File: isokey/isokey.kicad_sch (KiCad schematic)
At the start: 77 parts, among them Q1 BSS138, U1 BlackPill_STLINK, U3 TLV73318PDBV

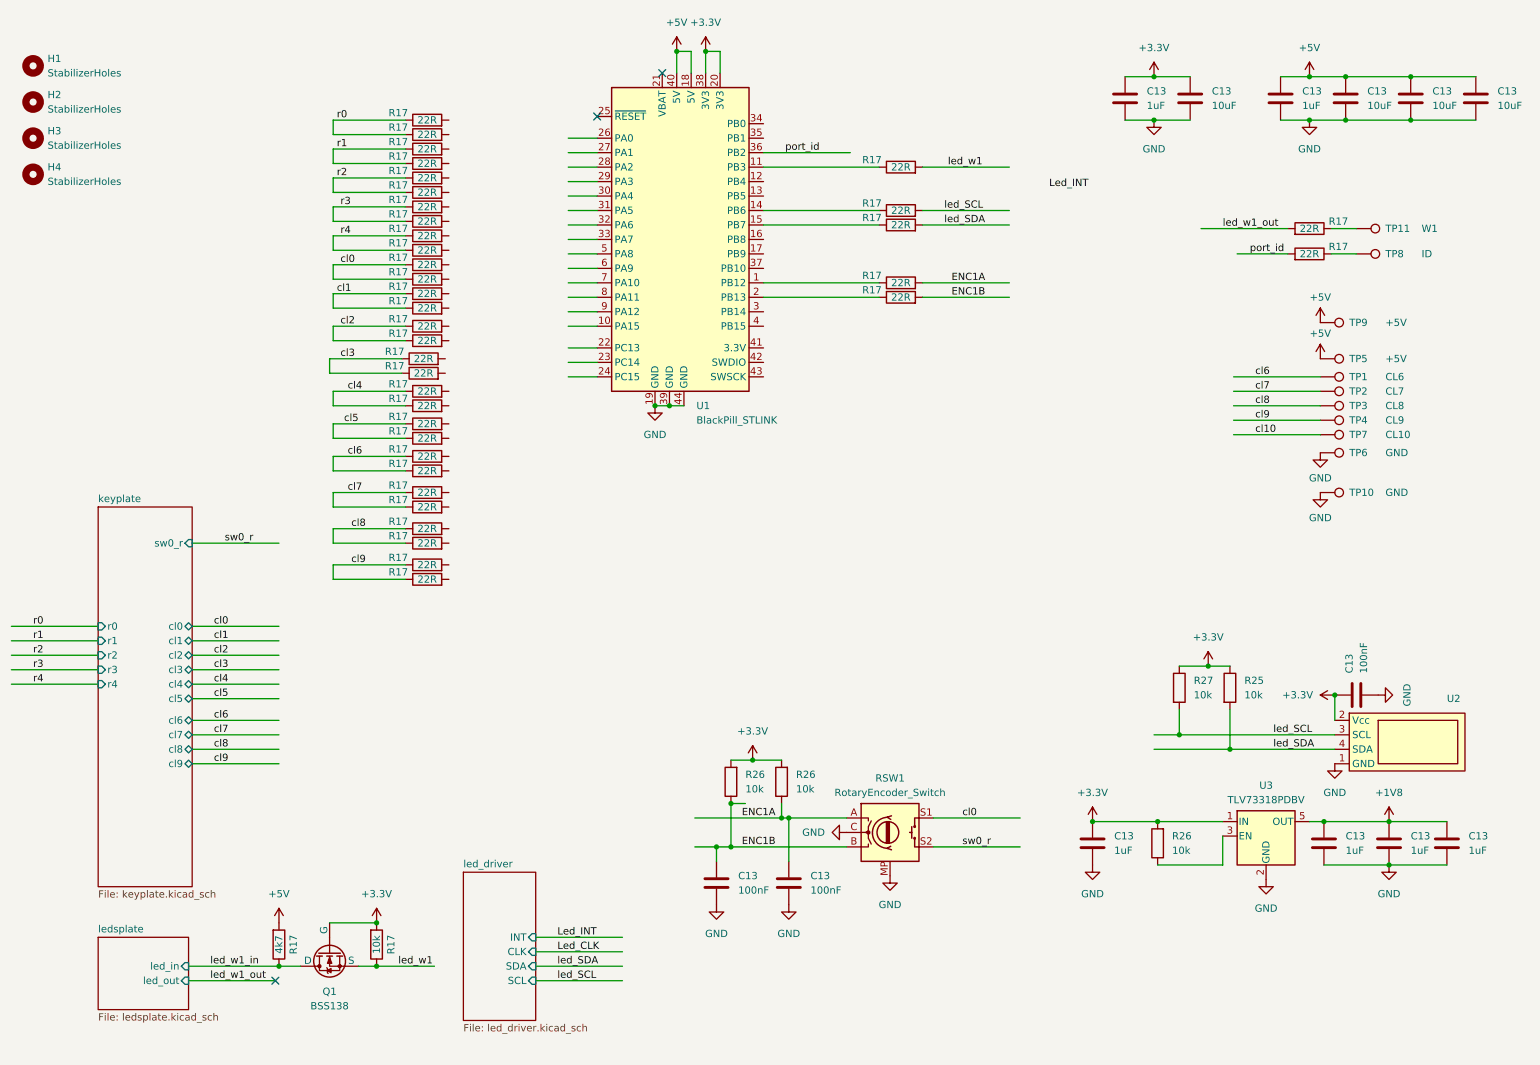
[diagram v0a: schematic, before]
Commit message: Continue routing
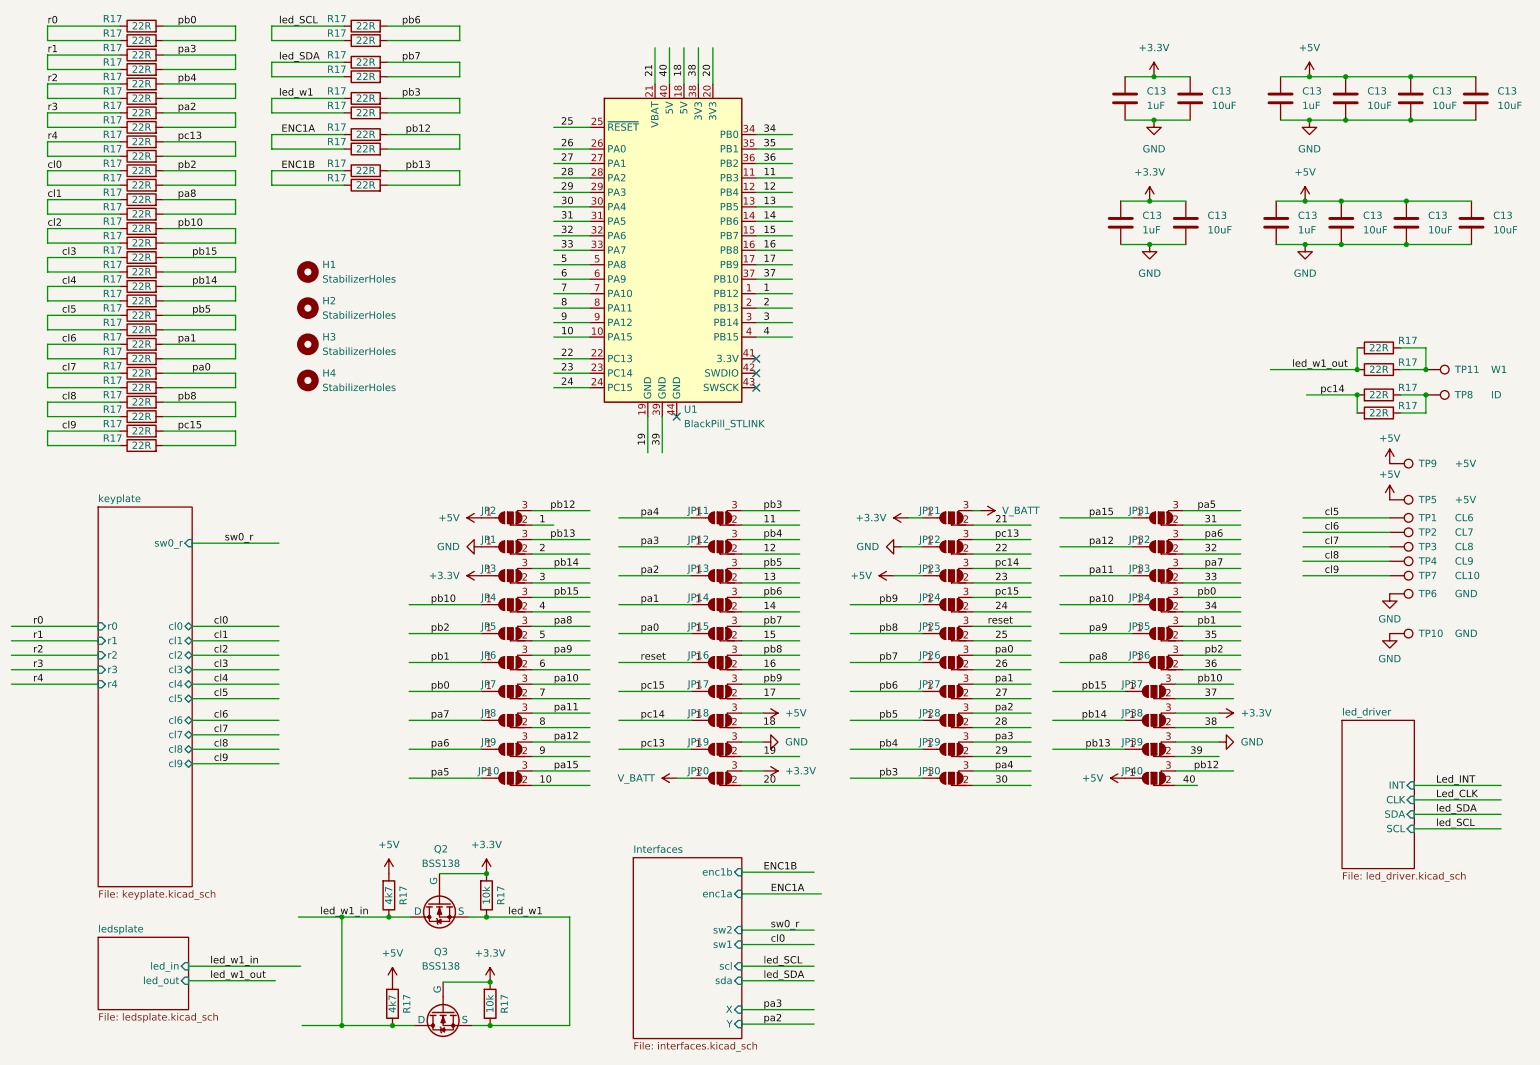
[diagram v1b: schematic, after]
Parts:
- removed C13 (x4): 1uF, Capacitor_SMD:C_0805_2012Metric, symbol Device:C
- removed C13 (x3): 100nF, Capacitor_SMD:C_0603_1608Metric_Pad1.08x0.95mm_HandSolder, symbol Device:C
- removed Q1: BSS138, Package_TO_SOT_SMD:SOT-23-3, symbol Simulation_SPICE:NMOS
- removed R17 (x4): 22R, Resistor_SMD:R_0603_1608Metric_Pad0.98x0.95mm_HandSolder, symbol Device:R
- removed R17: 4k7, Resistor_SMD:R_0603_1608Metric_Pad0.98x0.95mm_HandSolder, symbol Device:R
- removed R17, R25, R26 (x3), R27: 10k, Resistor_SMD:R_0603_1608Metric_Pad0.98x0.95mm_HandSolder, symbol Device:R
- removed RSW1: RotaryEncoder_Switch, Rotary_Encoder:RotaryEncoder_Alps_EC12E-Switch_Vertical_H20mm_CircularMountingHoles, symbol Device:RotaryEncoder_Switch
- removed U2: ~, Display:OLED_Display_128x32_SSD1306_i2c, symbol Display_Graphic:OLED_Display_128x32_SSD1306_i2c
- removed U3: TLV73318PDBV, Package_TO_SOT_SMD:SOT-23-5, symbol Regulator_Linear:TLV73318PDBV
- added C13 (x4): 10uF, Capacitor_SMD:C_1206_3216Metric, symbol Device:C
- added C13 (x2): 1uF, Capacitor_SMD:C_0805_2012Metric, symbol Device:C
- added JP1, JP10, JP11, JP12, JP13, JP14, JP15, JP16, JP17, JP18, JP19, JP2, JP20, JP21, JP22, JP23, JP24, JP25, JP26, JP27, JP28, JP29, JP3, JP30, JP31, JP32, JP33, JP34, JP35, JP36, JP37, JP38, JP39, JP4, JP40, JP5, JP6, JP7, JP8, JP9: SolderJumper_3_Open_line, Jumper:SolderJumper-3_P2.0mm_Open_TrianglePad1.0x1.5mm_NumberLabels, symbol Jumper:SolderJumper_3_Open_line
- added Q2, Q3: BSS138, Package_TO_SOT_SMD:SOT-23-3, symbol Simulation_SPICE:NMOS
- added R17 (x11): 22R, Resistor_SMD:R_0603_1608Metric_Pad0.98x0.95mm_HandSolder, symbol Device:R
- added R17 (x2): 4k7, Resistor_SMD:R_0603_1608Metric_Pad0.98x0.95mm_HandSolder, symbol Device:R
- added R17 (x2): 10k, Resistor_SMD:R_0603_1608Metric_Pad0.98x0.95mm_HandSolder, symbol Device:R
- U1: footprint Module:BlackPill_doble_top-bot -> Module:BlackPill
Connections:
- net cl10 is gone; now on net cl9: TP7.1
- net +3.3V: now also C13.1, C13.1, JP20.3 (B), JP21.1 (A), JP3.1 (A), JP38.3 (B), Q2.2 (G), Q3.2 (G), R17.2, R17.2; no longer U1.20 (3V3), U1.38 (3V3)
- net +5V: now also C13.1, C13.1, C13.1, C13.1, JP18.3 (B), JP2.1 (A), JP23.1 (A), JP40.1 (A), R17.2, R17.2; no longer U1.18 (5V), U1.40 (5V)
- net ENC1A: now also R17.1, R17.1
- net ENC1B: now also R17.1, R17.1
- net GND: now also C13.2, C13.2, C13.2, C13.2, C13.2, C13.2, JP1.1 (A), JP19.3 (B), JP22.1 (A), JP39.3 (B); no longer U1.19 (GND), U1.39 (GND), U1.44 (GND)
- net cl5: now also TP1.1
- net cl6: now also TP2.1; no longer TP1.1
- net cl7: now also TP3.1; no longer TP2.1
- net cl8: now also TP4.1; no longer TP3.1
- net cl9: no longer TP4.1
- net led_SCL: now also R17.1, R17.1
- net led_SDA: now also R17.1, R17.1
- net led_w1: now also R17.1, Q2.3 (S), Q3.3 (S), R17.1, R17.1, R17.1; no longer R17.2
- net led_w1_in: now also Q2.1 (D), Q3.1 (D), R17.1, R17.1
- net led_w1_out: now also R17.2
- net pc15: now reaches R17.2
- net pc15: now also R17.2, JP17.1 (A), JP24.3 (B)
- net at R17.1, TP8.1: now also R17.1
- net pa8: now reaches R17.2
- net pa8: now also R17.2, JP36.1 (A), JP5.3 (B)
- net pb14: now reaches R17.2
- net pb14: now also R17.2, JP3.3 (B), JP38.1 (A)
- net 2: now reaches U1.2 (PB13)
- net 2: now also JP1.2 (C)
- net pb0: now reaches R17.2
- net pb0: now also R17.2, JP34.3 (B), JP7.1 (A)
- net pb2: now reaches R17.2
- net pb2: now also R17.2, JP36.3 (B), JP5.1 (A)
- net pa1: now reaches R17.2
- net pa1: now also R17.2, JP14.1 (A), JP27.3 (B)
- net pb15: now reaches R17.2
- net pb15: now also R17.2, JP37.1 (A), JP4.3 (B)
- net 14: now reaches U1.14 (PB6)
- net 14: now also JP14.2 (C)
- net pb8: now reaches R17.2
- net pb8: now also R17.2, JP16.3 (B), JP25.1 (A)
- net 15: now reaches U1.15 (PB7)
- net 15: now also JP15.2 (C)
- net pb4: now reaches R17.2
- net pb4: now also R17.2, JP12.3 (B), JP29.1 (A)
- net pb5: now reaches R17.2
- net pb5: now also R17.2, JP13.3 (B), JP28.1 (A)
- net pa2: now reaches R17.2
- net pa2: now also R17.2, JP13.1 (A), JP28.3 (B)
- net pc13: now reaches R17.2
- net pc13: now also R17.2, JP19.1 (A), JP22.3 (B)
- net at R17.1, TP11.1: now also R17.1
- net 11: now reaches U1.11 (PB3)
- net 11: now also JP11.2 (C); no longer R17.1
- net pa0: now reaches R17.2
- net pa0: now also R17.2, JP15.1 (A), JP26.3 (B)
- net pb10: now reaches R17.2
- net pb10: now also R17.2, JP37.3 (B), JP4.1 (A)
- net pa3: now reaches R17.2
- net pa3: now also R17.2, JP12.1 (A), JP29.3 (B)
- net 1: now reaches U1.1 (PB12)
- net 1: now also JP2.2 (C)
- net 10: now reaches U1.10 (PA15)
- net 10: now also JP10.2 (C)
- net 12: now reaches U1.12 (PB4)
- net 12: now also JP12.2 (C)
- net 13: now reaches U1.13 (PB5)
- net 13: now also JP13.2 (C)
- net 16: now reaches U1.16 (PB8)
- net 16: now also JP16.2 (C)
- net 17: now reaches U1.17 (PB9)
- net 17: now also JP17.2 (C)
- net 21: now reaches U1.21 (VBAT)
- net 21: now also JP21.2 (C)
- net 22: now reaches U1.22 (PC13)
- net 22: now also JP22.2 (C)
- net 23: now reaches U1.23 (PC14)
- net 23: now also JP23.2 (C)
- net 24: now reaches U1.24 (PC15)
- net 24: now also JP24.2 (C)
- net 25: now reaches U1.25 (~{RESET})
- net 25: now also JP25.2 (C)
- net 26: now reaches U1.26 (PA0)
- net 26: now also JP26.2 (C)
- net 27: now reaches U1.27 (PA1)
- net 27: now also JP27.2 (C)
- net 28: now reaches U1.28 (PA2)
- net 28: now also JP28.2 (C)
- net 29: now reaches U1.29 (PA3)
- net 29: now also JP29.2 (C)
- net 3: now reaches U1.3 (PB14)
- net 3: now also JP3.2 (C)
- net 30: now reaches U1.30 (PA4)
- net 30: now also JP30.2 (C)
- net 31: now reaches U1.31 (PA5)
- net 31: now also JP31.2 (C)
- net 32: now reaches U1.32 (PA6)
- net 32: now also JP32.2 (C)
- net 33: now reaches U1.33 (PA7)
- net 33: now also JP33.2 (C)
- net 34: now reaches U1.34 (PB0)
- net 34: now also JP34.2 (C)
- net 35: now reaches U1.35 (PB1)
- net 35: now also JP35.2 (C)
- net 37: now reaches U1.37 (PB10)
- net 37: now also JP37.2 (C)
- net 4: now reaches U1.4 (PB15)
- net 4: now also JP4.2 (C)
- net 5: now reaches U1.5 (PA8)
- net 5: now also JP5.2 (C)
- net 6: now reaches U1.6 (PA9)
- net 6: now also JP6.2 (C)
- net 7: now reaches U1.7 (PA10)
- net 7: now also JP7.2 (C)
- net 8: now reaches U1.8 (PA11)
- net 8: now also JP8.2 (C)
- net 9: now reaches U1.9 (PA12)
- net 9: now also JP9.2 (C)
- net port_id renamed 36
- net 36: now also JP36.2 (C); no longer R17.2
- new net 18: JP18.2 (C), U1.18 (5V)
- new net 19: JP19.2 (C), U1.19 (GND)
- new net 20: JP20.2 (C), U1.20 (3V3)
- new net 38: JP38.2 (C), U1.38 (3V3)
- new net 39: JP39.2 (C), U1.39 (GND)
- new net 40: JP40.2 (C), U1.40 (5V)
- new net V_BATT: JP20.1 (A), JP21.3 (B)
- new net pa10: JP34.1 (A), JP7.3 (B)
- new net pa11: JP33.1 (A), JP8.3 (B)
- new net pa12: JP32.1 (A), JP9.3 (B)
- new net pa15: JP10.3 (B), JP31.1 (A)
- new net pa4: JP11.1 (A), JP30.3 (B)
- new net pa5: JP10.1 (A), JP31.3 (B)
- new net pa6: JP32.3 (B), JP9.1 (A)
- new net pa7: JP33.3 (B), JP8.1 (A)
- new net pa9: JP35.1 (A), JP6.3 (B)
- new net pb1: JP35.3 (B), JP6.1 (A)
- new net pb12: JP2.3 (B), JP40.3 (B), R17.2, R17.2
- new net pb13: JP1.3 (B), JP39.1 (A), R17.2, R17.2
- new net pb3: JP11.3 (B), JP30.1 (A), R17.2, R17.2
- new net pb6: JP14.3 (B), JP27.1 (A), R17.2, R17.2
- new net pb7: JP15.3 (B), JP26.1 (A), R17.2, R17.2
- new net pb9: JP17.3 (B), JP24.1 (A)
- new net pc14: JP18.1 (A), JP23.3 (B), R17.2, R17.2
- new net reset: JP16.1 (A), JP25.3 (B)
- no-connect marks 3 -> 4
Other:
- added sheet Interfaces (interfaces.kicad_sch)
- moved on the sheet: H1, H2, H3, H4, R17, TP1, TP10, TP11, TP2, TP3, TP4, TP5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
